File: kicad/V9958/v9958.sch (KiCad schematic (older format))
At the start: 26 parts, among them J1 Conn_01x01, J2 Conn_01x01, J3 Conn_01x04, J4 Conn_01x04, Q1 BC547, Q2 BC547, Q3 BC547, Q4 BC547, U1 7400, U2 V9958, U3 DRAM_64KX4, U4 DRAM_64KX4, U5 DRAM_64KX4, U6 DRAM_64KX4, Y1 21,443Mhz

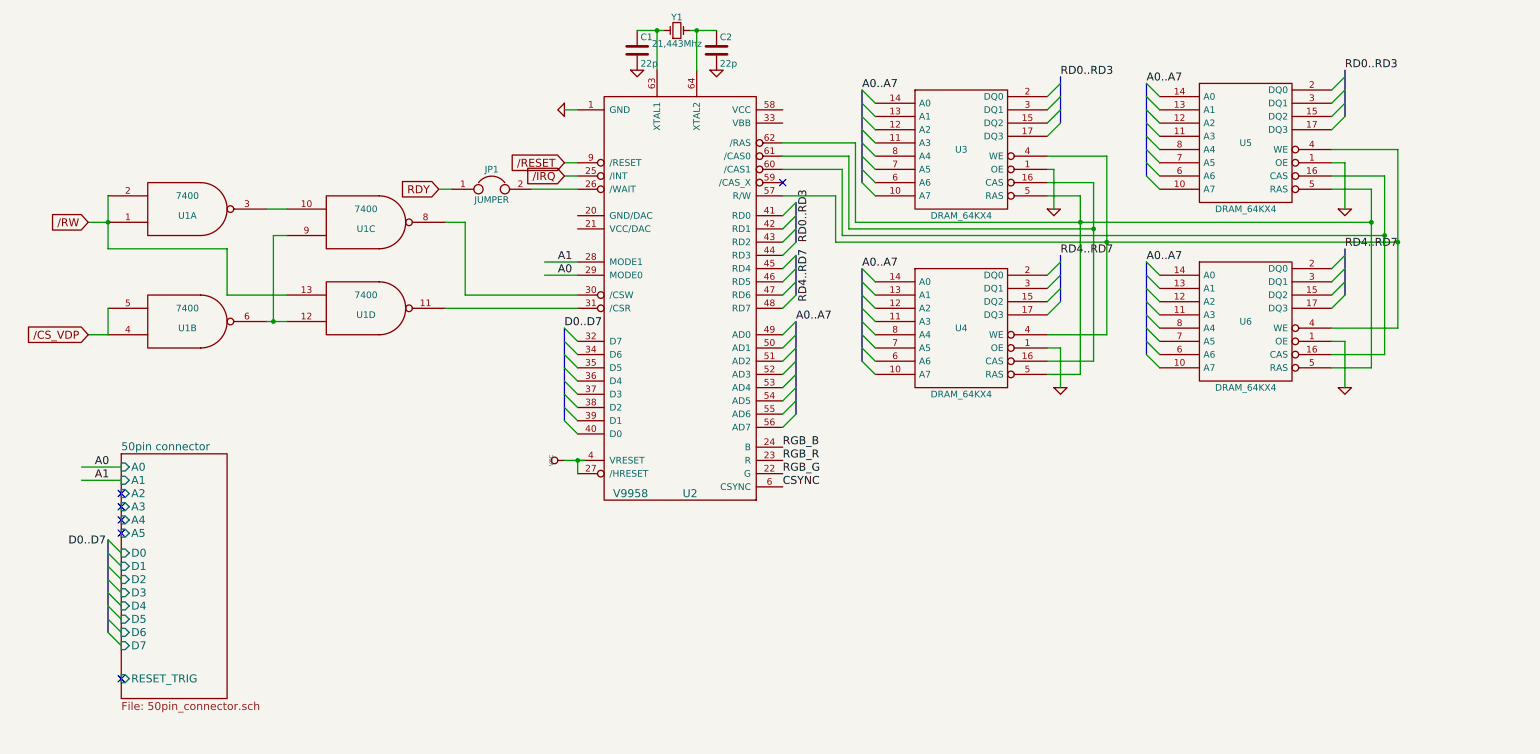
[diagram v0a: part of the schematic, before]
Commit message: cleanup, fixes
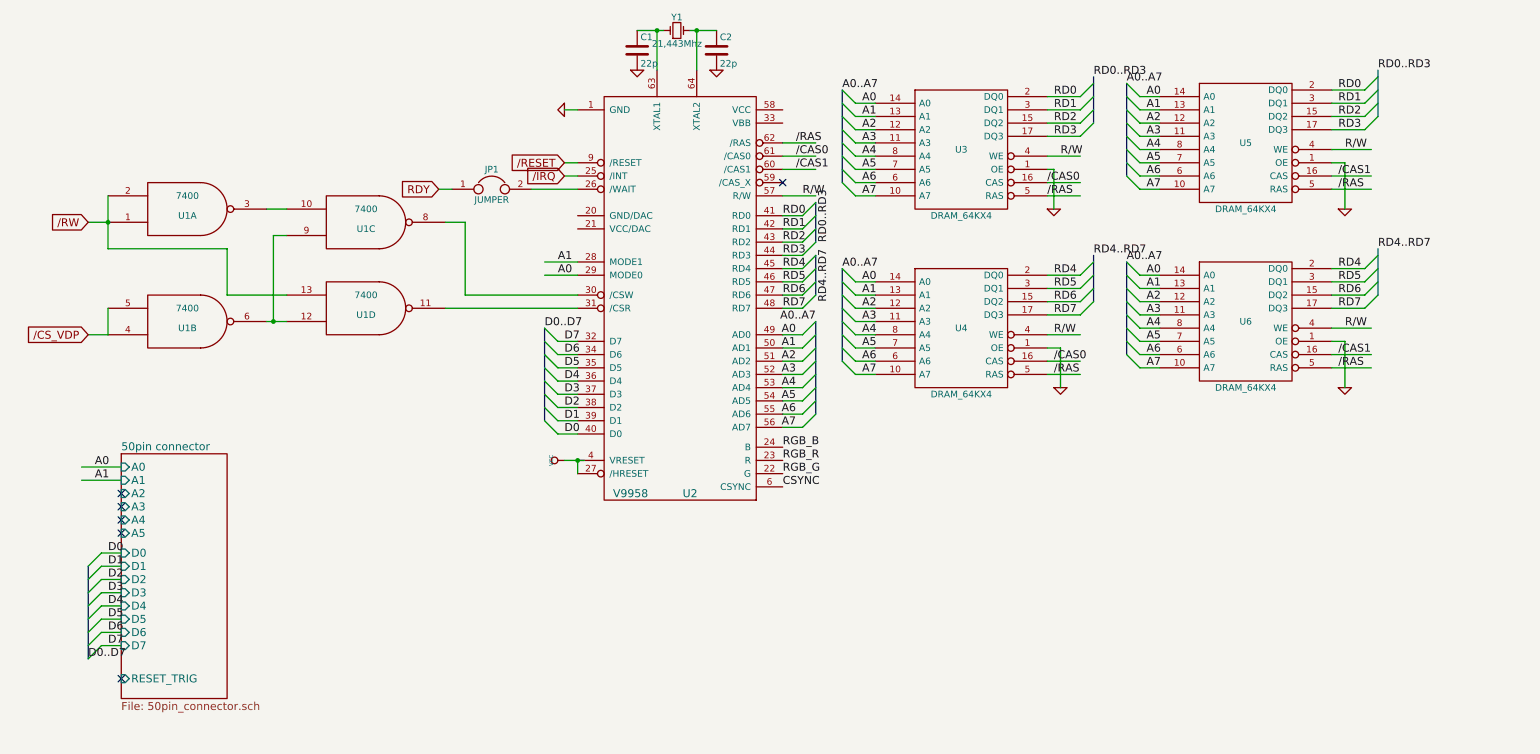
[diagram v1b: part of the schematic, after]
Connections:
- net labels added: /CAS0, /CAS1, /RAS, A2, A3, A4, A5, A6, A7, D0, D1, D2, D3, D4, D5, D6, D7, R/W, RD0, RD1, RD2, RD3, RD4, RD5, RD6, RD7
- wire segments 114 -> 180
